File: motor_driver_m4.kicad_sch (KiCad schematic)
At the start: 31 parts, among them J13 Conn_01x01_Pin, J14 Conn_01x01_Pin, J15 Conn_01x01_Pin, M4 DRV8320SRTVR, Q19 NP80N06D6, Q20 NP80N06D6, Q21 NP80N06D6, Q22 NP80N06D6, Q23 NP80N06D6, Q24 NP80N06D6

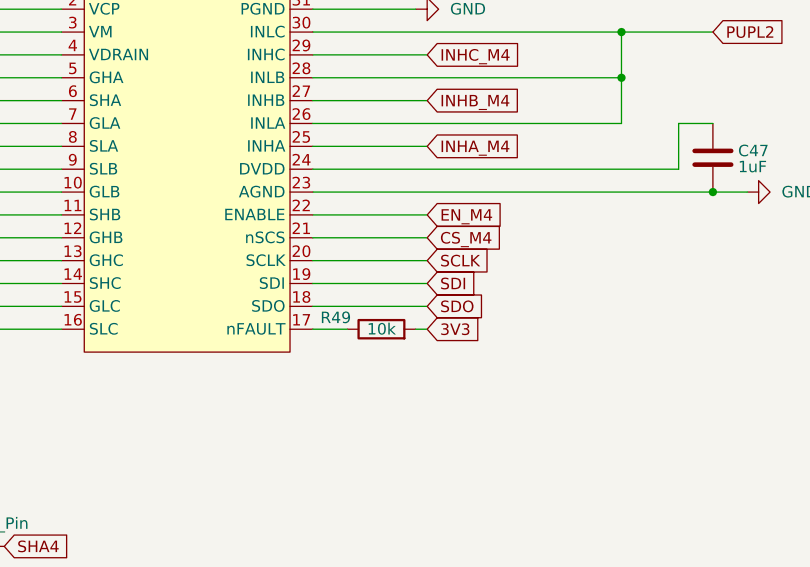
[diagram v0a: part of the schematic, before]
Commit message: ...
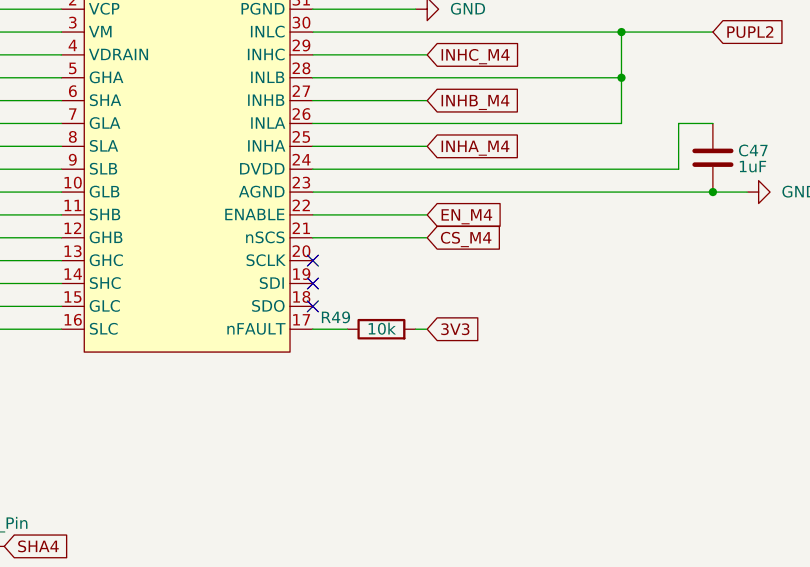
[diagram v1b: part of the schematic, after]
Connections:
- net SCLK: no longer names the net of M4.20 (SCLK)
- net SDI: no longer names the net of M4.19 (SDI)
- net SDO: no longer names the net of M4.18 (SDO)
- no-connect marks 0 -> 3
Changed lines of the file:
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@@
 		(color 0 0 0 0)
 	)
+	(no_connect
+		(at 92.71 80.01)
+	)
+	(no_connect
+		(at 92.71 77.47)
+	)
+	(no_connect
+		(at 92.71 74.93)
+	)
 	(wire
 		(pts
@@
 	(wire
 		(pts
-			(xy 105.41 74.93) (xy 92.71 74.93)
-		)
-		(stroke
-			(width 0)
-			(type default)
-		)
-	)
-	(wire
-		(pts
 			(xy 105.41 57.15) (xy 92.71 57.15)
 		)
@@
 	(wire
 		(pts
-			(xy 105.41 77.47) (xy 92.71 77.47)
-		)
-		(stroke
-			(width 0)
-			(type default)
-		)
-	)
-	(wire
-		(pts
 			(xy 219.71 36.83) (xy 231.14 36.83)
 		)
@@
 	(wire
 		(pts
-			(xy 92.71 80.01) (xy 105.41 80.01)
-		)
-		(stroke
-			(width 0)
-			(type default)
-		)
-	)
-	(wire
-		(pts
 			(xy 214.63 52.07) (xy 219.71 52.07)
 		)
@@
 		)
 	)
-	(global_label "SDI"
-		(shape input)
-		(at 105.41 77.47 0)
-		(fields_autoplaced yes)
-		(effects
-			(font
-				(size 1.27 1.27)
-			)
-			(justify left)
-		)
-		(property "Intersheetrefs" "${INTERSHEET_REFS}"
-			(at 111.4795 77.47 0)
-			(effects
-				(font
-					(size 1.27 1.27)
-				)
-				(justify left)
-				(hide yes)
-			)
-		)
-	)
 	(global_label "GHC4"
 		(shape input)
@@
 		)
 	)
-	(global_label "SDO"
-		(shape input)
-		(at 105.41 80.01 0)
-		(fields_autoplaced yes)
-		(effects
-			(font
-				(size 1.27 1.27)
-			)
-			(justify left)
-		)
-		(property "Intersheetrefs" "${INTERSHEET_REFS}"
-			(at 112.2052 80.01 0)
-			(effects
-				(font
-					(size 1.27 1.27)
-				)
-				(justify left)
-				(hide yes)
-			)
-		)
-	)
 	(global_label "GHA4"
 		(shape input)
@@
 			(effects
 				(font
-					(size 1.27 1.27)
-				)
-				(justify left)
-				(hide yes)
-			)
-		)
-	)
-	(global_label "SCLK"
-		(shape input)
-		(at 105.41 74.93 0)
-		(fields_autoplaced yes)
-		(effects
-			(font
-				(size 1.27 1.27)
-			)
-			(justify left)
-		)
-		(property "Intersheetrefs" "${INTERSHEET_REFS}"
-			(at 113.1728 74.93 0)
-			(effects
-				(font
